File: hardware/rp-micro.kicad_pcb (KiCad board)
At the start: 2 copper layers, 17.8 x 33 mm, 44 parts, among them J1 USB_C_Receptacle_USB2.0, J2 Conn_01x12, J3 Conn_01x12, J4 Conn_01x05, SW1 BOOT, SW2 RESET, U1 RT9013-33GB, U2 W25Q64JVXGIQ, U3 RP2040, Y1 12MHz

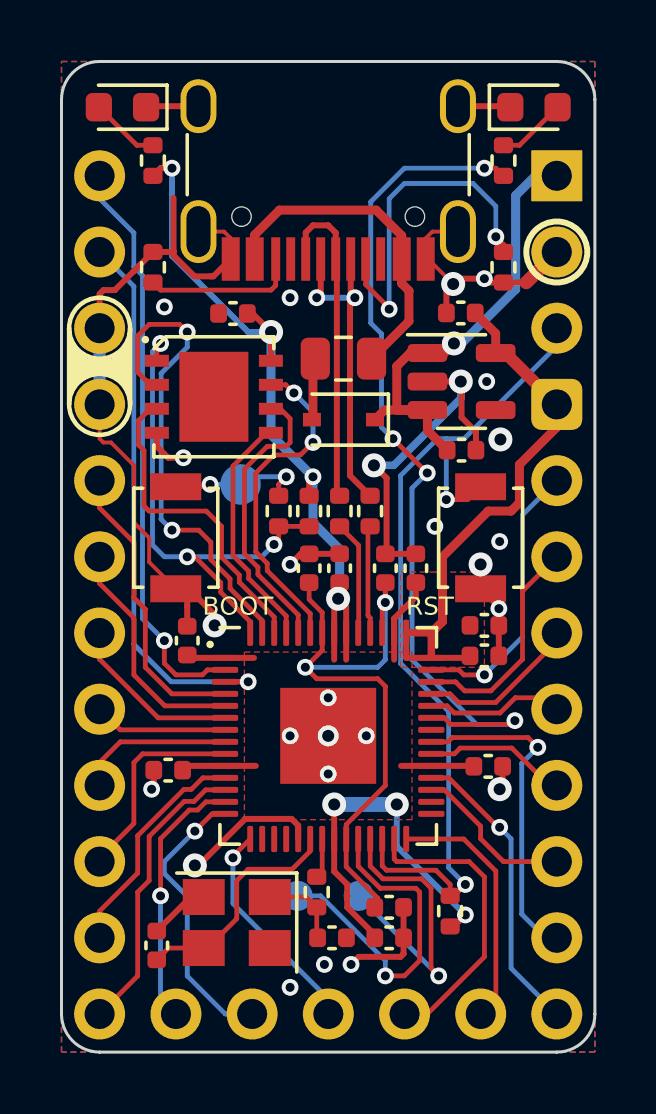
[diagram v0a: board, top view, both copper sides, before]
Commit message: rev 1.1 completed
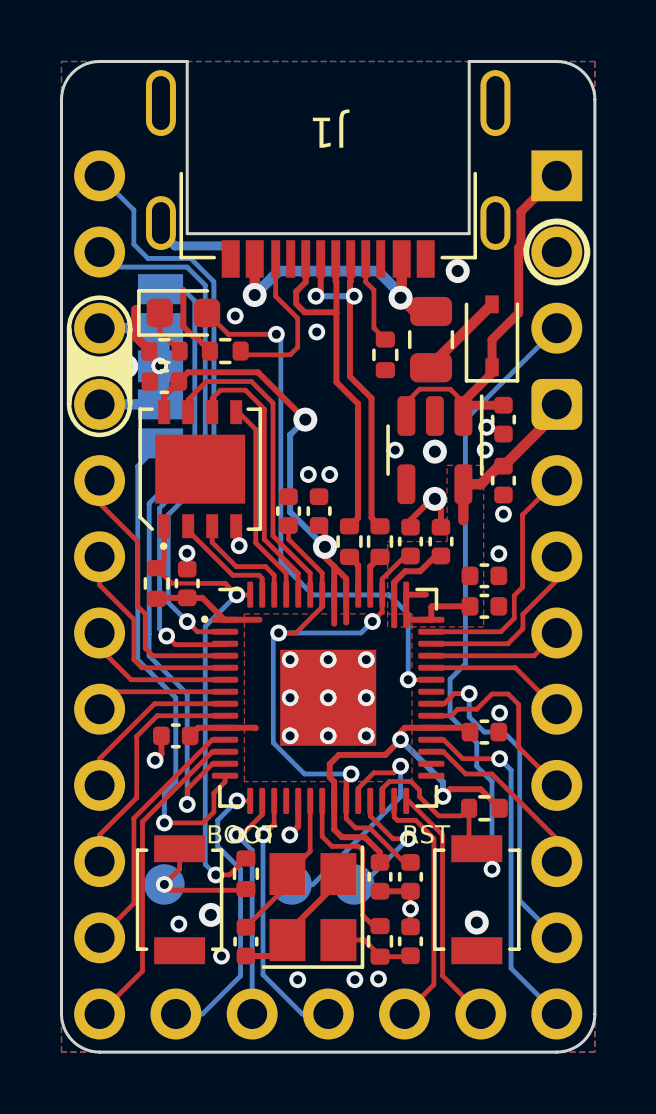
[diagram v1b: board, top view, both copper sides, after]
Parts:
- removed the LD1 at (132.8, 58.7)
- removed the R3 at (133.9, 60.5)
- removed kibuzzard-6360A6AE: G***, kibuzzard-6360A6AE
- added JP1: SolderJumper_3_Bridged12, Jumper:SolderJumper-3_P1.3mm_Bridged12_Pad1.0x1.5mm, B.Cu at (134.1, 66.0)
- added JP2: SolderJumper_3_Bridged12, Jumper:SolderJumper-3_P1.3mm_Bridged12_Pad1.0x1.5mm, B.Cu at (134.1, 68.6)
- added kibuzzard-637CA201: G***, kibuzzard-637CA201, B.Cu at (137.9, 81.1)
- J1: footprint rp-micro:USB_C_Receptacle_TYPE-C-31-M-12 -> rp-micro:USB Type-C Mid-Mount Receptacle 16P
- TP1: renamed from TP2; footprint TestPoint:TestPoint_Pad_D1.0mm -> TestPoint:TestPoint_Pad_D2.0mm
- TP2: renamed from TP3; footprint TestPoint:TestPoint_Pad_D1.0mm -> TestPoint:TestPoint_Pad_D2.0mm
- moved TP3 13.6 mm to (134.2, 84.6)
- moved LD1 13.5 mm to (134.9, 65.5)
- moved R9 13.0 mm to (134.2, 66.8), turned to 180 degrees
- moved R4 12.1 mm to (137.0, 84.2), turned to 90 degrees
- moved SW1 12.1 mm to (134.7, 85.1)
- moved SW2 12.1 mm to (144.7, 85.1)
- moved C15 5.77 mm to (145.5, 71.1), turned to -90 degrees
- moved D1 5.69 mm to (145.2, 66.3), turned to 90 degrees
- moved R5 5.62 mm to (134.0, 74.5), turned to 90 degrees
- moved R6 4.90 mm to (141.6, 66.9)
- moved R7 3.69 mm to (136.3, 66.8), turned to 180 degrees
- moved R8 3.61 mm to (144.9, 82.0), turned to 180 degrees
- moved C16 3.22 mm to (134.2, 67.8)
- moved F1 2.99 mm to (143.1, 66.4), turned to -90 degrees
- moved C3 2.97 mm to (137.0, 86.5), turned to 90 degrees
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- renumbered C6 to C1, C13 to C10, C14 to C11, C15 to C12, C16 to C13, C1 to C14, C2 to C15, C3 to C16, C9 to C2, C4 to C3, C5 to C4, C7 to C5, C10 to C6, C8 to C7, C11 to C8, C12 to C9, J4 to J3, J3 to J4, LD2 to LD1, R4 to R1, R5 to R2, R8 to R3, R7 to R4, R6 to R5, R1 to R6, R2 to R7, R9 to R8, R10 to R9, TP1 to TP3, U3 to U1, U1 to U3
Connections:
- net 22_SLCK renamed 22_SCLK
- net Net-(R4-Pad2) renamed /RPD+
- net Net-(R5-Pad2) renamed /RPD-
- net QSPI_0 renamed QSPI_D0
- net QSPI_1 renamed QSPI_D1
- net QSPI_2 renamed QSPI_D2
- net QSPI_3 renamed QSPI_D3
- D1 pad 2: VBUS -> +5V
- F1 pad 1: Net-(F1-Pad1) -> VBUS
- F1 pad 2: VBUS -> +5V
- J1 pad A4: Net-(F1-Pad1) -> VBUS
- J1 pad A9: Net-(F1-Pad1) -> VBUS
- J1 pad B4: Net-(F1-Pad1) -> VBUS
- J1 pad B9: Net-(F1-Pad1) -> VBUS
- J2 pad 3: GND -> Net-(J2-Pad3)
- J2 pad 4: GND -> Net-(J2-Pad4)
- J3 pad 1: 10 -> 12
- J3 pad 2: 11 -> 13
- J3 pad 3: 12 -> 14
- LD1 pad 1: GND -> Net-(LD1-Pad1)
- LD1 pad 2: Net-(LD2-Pad2) -> STATE_LED
- R9 pad 1: STATE_LED -> Net-(LD1-Pad1)
- R9 pad 2: Net-(LD2-Pad2) -> GND
- U1 pad 16: unconnected-(U3-Pad16) -> 13
- U1 pad 17: unconnected-(U3-Pad17) -> 14
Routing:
- net GND: track 65.1 -> 20.4 mm, vias 26 -> 36
- net +3V3: track 66.9 -> 50.1 mm, vias 7 -> 4
- net 10: track 8.71 -> 21.4 mm
- net QSPI_D1: track 16.2 -> 3.89 mm, vias 2 -> 0
- net Net-(F1-Pad1): track 11.1 -> 0.00 mm
- net STATE_LED: track 28.6 -> 18.2 mm, vias 4 -> 2
- net 14: track 0.00 -> 8.67 mm, vias 0 -> 1
- net Net-(J1-PadA5): track 11.4 -> 3.16 mm, vias 2 -> 0
- net 13: track 0.00 -> 7.77 mm, vias 0 -> 1
- net VBUS: track 2.08 -> 9.75 mm, vias 0 -> 2
- net 11: track 9.50 -> 16.8 mm
- net QSPI_D2: track 10.8 -> 3.79 mm
- net SWDIO: track 10.0 -> 4.52 mm
- net Net-(R3-Pad2): track 1.33 -> 5.62 mm
- net ~{RESET}: track 29.9 -> 26.5 mm, vias 2 -> 1
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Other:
- outline, holes or cut-outs redrawn
- board text added: "13"
- board text added: "14"
